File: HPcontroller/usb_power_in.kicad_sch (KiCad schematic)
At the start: 13 parts, among them J2 USB_C_Receptacle, Q2 AON7410, U8 IP2721

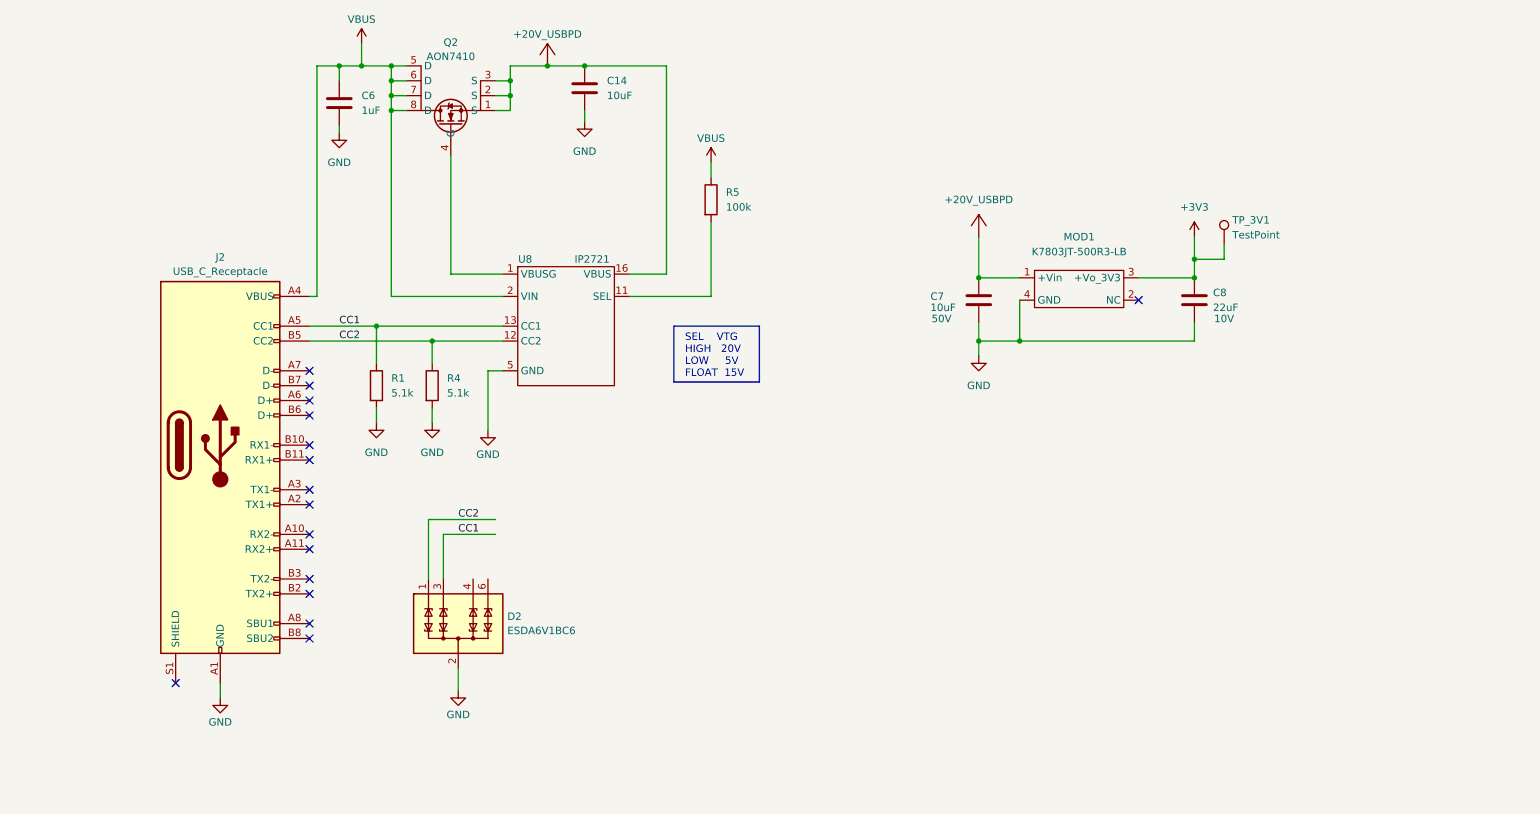
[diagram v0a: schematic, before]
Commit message: v3 routing
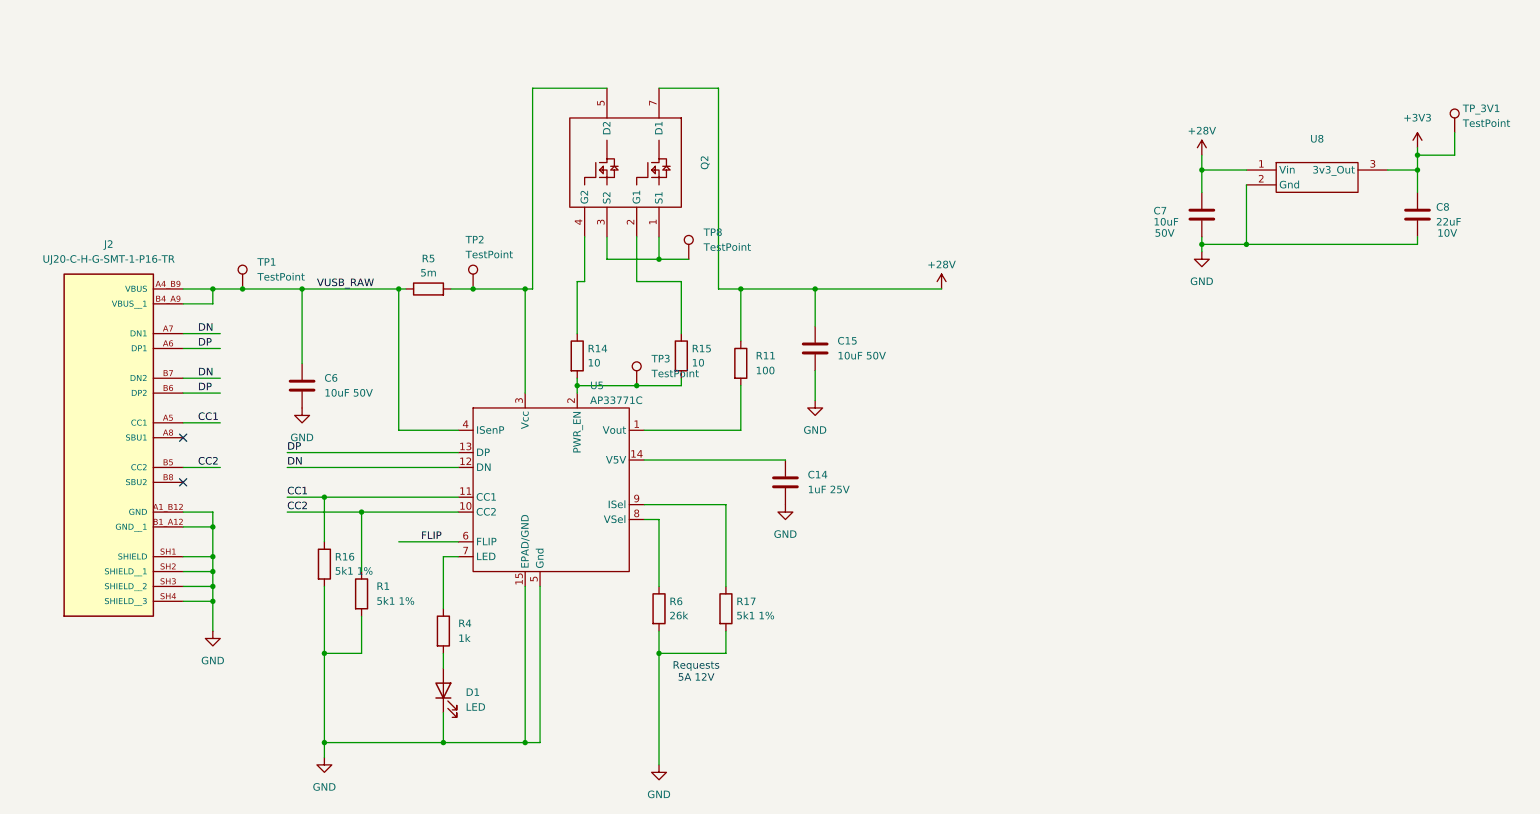
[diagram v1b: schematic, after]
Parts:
- removed D2: ESDA6V1BC6, Package_TO_SOT_SMD:SOT-23-6, symbol Power_Protection:ESDA6V1BC6
- removed J2: USB_C_Receptacle, Connector_USB:USB_C_Receptacle_JAE_DX07S016JA1R1500, symbol Connector:USB_C_Receptacle
- removed MOD1: K7803JT-500R3-LB, HPfootprint:MORNSUN_K7803JT-500R3-LB, symbol PDHV_sym:K7803JT-500R3-LB
- removed Q2: AON7410, HPfootprint:DFN3X3A_8L_EPA1_P_AOS, symbol PDHV_sym:AON7410
- removed U8: IP2721, Package_SO:TSSOP-16_4.4x5mm_P0.65mm, symbol project_assorted:IP2721
- added C15: 10uF 50V, Capacitor_SMD:C_1206_3216Metric_Pad1.33x1.80mm_HandSolder, symbol Device:C
- added D1: LED, LED_SMD:LED_0603_1608Metric_Pad1.05x0.95mm_HandSolder, symbol Device:LED
- added J2: UJ20-C-H-G-SMT-1-P16-TR, hotplate_Library:SAMESKY_UJ20-C-H-G-SMT-1-P16-TR, symbol mpssym:UJ20-C-H-G-SMT-1-P16-TR
- added Q2: ~, hotplate_Library:LFPAK56D, symbol Hotplate_Library:BUK9K25-40RAX
- added R11: 100, Resistor_SMD:R_0402_1005Metric_Pad0.72x0.64mm_HandSolder, symbol Device:R
- added R14, R15: 10, Resistor_SMD:R_0402_1005Metric_Pad0.72x0.64mm_HandSolder, symbol Device:R
- added R16, R17: 5k1 1%, Resistor_SMD:R_0402_1005Metric_Pad0.72x0.64mm_HandSolder, symbol Device:R
- added R6: 26k, Resistor_SMD:R_0603_1608Metric_Pad0.98x0.95mm_HandSolder, symbol Device:R
- added TP1, TP2, TP3, TP8: TestPoint, TestPoint:TestPoint_Pad_D1.5mm, symbol Connector:TestPoint
- added U5: AP33771C, Package_DFN_QFN:DFN-14-1EP_3x3mm_P0.4mm_EP1.78x2.35mm, symbol C_buck_syms:AP33771C
- added U8: ~, hotplate_Library:D78B33-0.5, symbol Hotplate_Library:D78B33-0.5
- C14: value 10uF -> 1uF 25V; footprint Capacitor_SMD:C_0805_2012Metric -> Capacitor_SMD:C_0402_1005Metric_Pad0.74x0.62mm_HandSolder; Digikey PN 490-18663-1-ND -> (none); MPN GRM21BR61H106KE43L -> 0402X105K250CT; Voltage 50V -> (none)
- C6: value 1uF -> 10uF 50V; footprint Capacitor_SMD:C_0603_1608Metric -> Capacitor_SMD:C_1206_3216Metric_Pad1.33x1.80mm_HandSolder; Digikey PN 587-2400-1-ND -> (none); MPN UMK107BJ105KA-T -> CL31A106KBHNNNE; Voltage 25V -> (none)
- R1: value 5.1k -> 5k1 1%; footprint Resistor_SMD:R_0603_1608Metric -> Resistor_SMD:R_0402_1005Metric_Pad0.72x0.64mm_HandSolder; Digikey PN RMCF0603FT5K10CT-ND -> (none); MPN RMCF0603FT5K10 -> RC0402FR-135K1L; Tol 1% -> (none)
- R4: value 5.1k -> 1k; footprint Resistor_SMD:R_0603_1608Metric -> Resistor_SMD:R_0402_1005Metric_Pad0.72x0.64mm_HandSolder; Digikey PN RMCF0603FT5K10CT-ND -> (none); MPN RMCF0603FT5K10 -> RC0402FR-071KL; Tol 1% -> (none)
- R5: value 100k -> 5m; footprint Resistor_SMD:R_0603_1608Metric -> Resistor_SMD:R_0603_1608Metric_Pad0.98x0.95mm_HandSolder; Digikey PN RMCF0603JG100KCT-ND -> (none); MPN RMCF0603JG100K -> PA0603FRE470R005L
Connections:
- net +3V3: now also U8.3 (3v3_Out)
- net CC1: now also J2.A5 (CC1), R16.1, U5.11 (CC1); no longer R1.1
- net CC2: now also R1.1, J2.B5 (CC2), U5.10 (CC2); no longer R4.1
- net GND: now also C15.2, D1.1 (K), J2.A1_B12 (GND), J2.B1_A12 (GND__1), J2.SH1 (SHIELD), J2.SH2 (SHIELD__1), J2.SH3 (SHIELD__2), J2.SH4 (SHIELD__3), R16.2, R17.2, R6.2, U5.15 (EPAD/GND), U5.5 (Gnd), U8.2 (Gnd); no longer R4.2
- net at R5.2: now also Q2.5 (D2), TP2.1, U5.3 (Vcc)
- net +20V_USBPD: no longer names the net of C14.1
- net +20V_USBPD: now also U5.14 (V5V); no longer C7.1
- net VBUS renamed VUSB_RAW
- net VUSB_RAW: now also J2.A4_B9 (VBUS), J2.B4_A9 (VBUS__1), TP1.1, U5.4 (ISenP)
- new net: R11.2, U5.1 (Vout)
- new net: R4.1, U5.7 (LED)
- new net: D1.2 (A), R4.2
- new net: R14.2, R15.2, TP3.1, U5.2 (PWR_EN)
- new net: R6.1, U5.8 (VSel)
- new net: R17.1, U5.9 (ISel)
- new net: Q2.4 (G2), R14.1
- new net: Q2.1 (S1), Q2.3 (S2), TP8.1
- new net: Q2.2 (G1), R15.1
- new net +28V: C15.1, C7.1, Q2.7 (D1), R11.1, U8.1 (Vin)
- new net DN: J2.A7 (DN1), J2.B7 (DN2), U5.12 (DN)
- new net DP: J2.A6 (DP1), J2.B6 (DP2), U5.13 (DP)
- new net FLIP: U5.6 (FLIP)
- no-connect marks 16 -> 2
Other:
- note added: "Requests 5A 12V"
- note removed: "SEL VTG HIGH 20V LOW 5V FLOAT 15V"
- moved on the sheet: C7, C8, TP_3V1
